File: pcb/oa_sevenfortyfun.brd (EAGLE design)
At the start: 88.9 x 63.4 mm, 45 parts, among them J1 1X01, J2 1X01, J3 1X01, J4 1X01, J5 1X01, J6 1X01, J7 1X01, J8 1X01, Q1 2N3904, Q10 2N3904, Q11 2N3904, Q12 2N3904, Q13 2N3904, Q14 2N3904, Q15 2N3906, Q16 2N3904, Q17 2N3906, Q18 2N3906, Q19 2N3906, Q2 2N3904, Q20 2N3906, Q3 2N3906, Q4 2N3906, Q5 2N3904, Q6 2N3904, Q7 2N3904, Q8 2N3904, Q9 2N3904

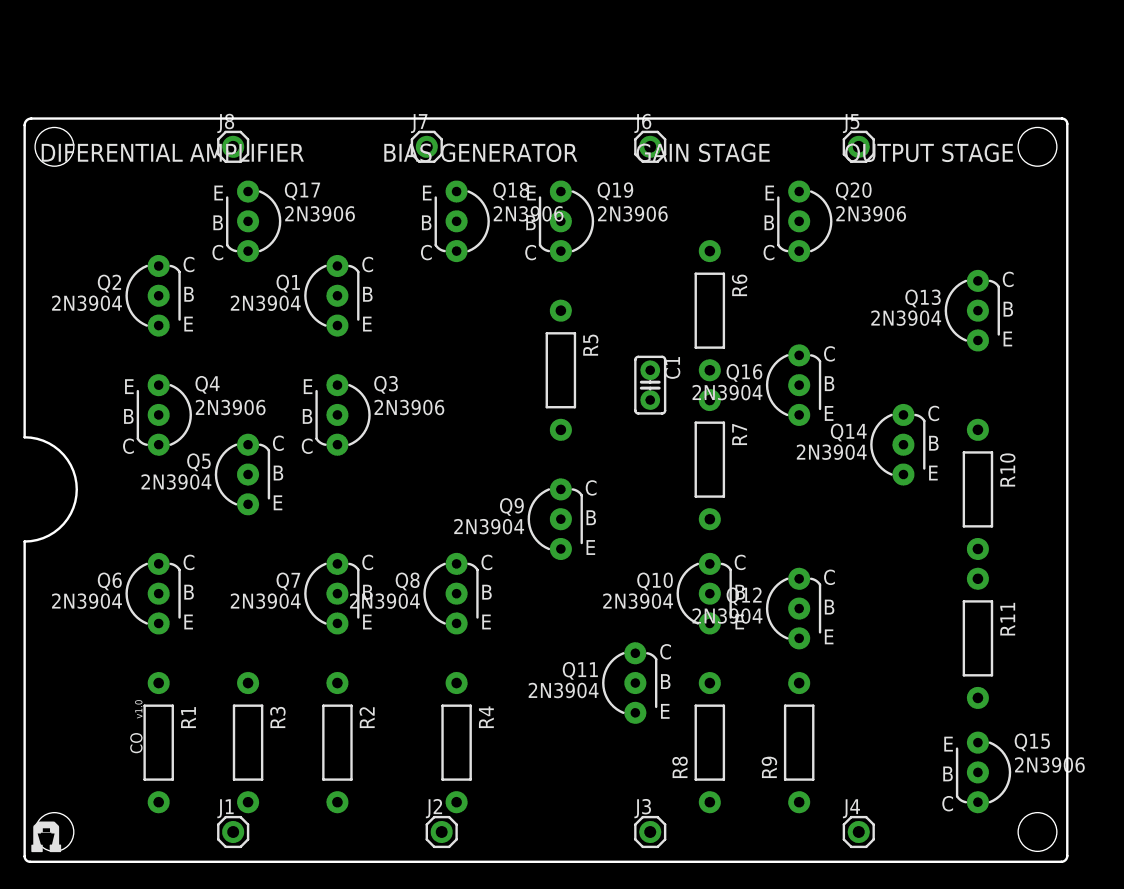
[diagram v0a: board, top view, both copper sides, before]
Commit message: Working on silkscreen
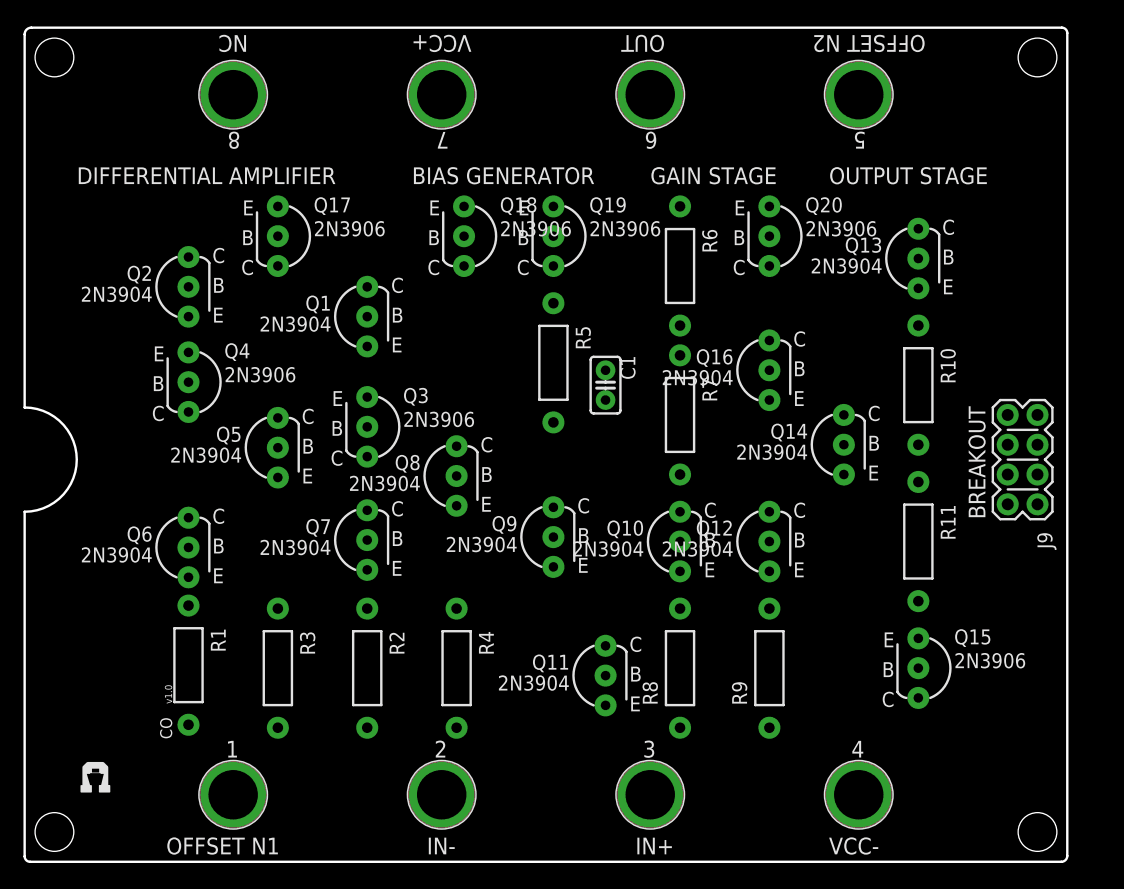
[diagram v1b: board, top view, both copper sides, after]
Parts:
- added J9: 2X04, Ai_Connectors:2X04
- J1, J2, J3, J4, J5, J6, J7, J8: value 1X01 -> 1X01-TERM; device Ai_Connectors:1X01 -> Ai_Connectors:1X01-TERM
- moved Q15 10.2 mm to (76.2, 16.5)
- moved R10 10.2 mm to (76.2, 40.6)
- moved Q8 10.0 mm to (36.8, 32.9)
- moved R11 9.69 mm to (76.2, 27.3)
- moved STANDOFF3 7.62 mm to (2.54, 68.6)
- moved STANDOFF4 7.62 mm to (86.4, 68.6)
- moved R1 7.08 mm to (14.0, 16.8)
- moved R9 6.84 mm to (63.5, 16.5)
- moved R2 6.84 mm to (29.2, 16.5)
- moved R3 6.84 mm to (21.6, 16.5)
- moved R8 6.84 mm to (55.9, 16.5)
- moved Q13 6.75 mm to (76.2, 51.4)
- moved U$3 6.59 mm to (4.70, 5.84)
- moved R4 6.35 mm to (36.8, 16.5)
- moved Q12 6.25 mm to (63.5, 27.3)
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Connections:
- net IN+: now also J9.5
- net IN-: now also J9.3
- net NC: now also J9.2
- net OFFSET_N1: now also J9.1
- net OFFSET_N2: now also J9.8
- net OUT: now also J9.6
- net VCC+: now also J9.4
- net VCC-: now also J9.7
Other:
- board size 88.9 x 63.4 mm -> 88.9 x 71.1 mm
- board text added: "1"
- board text added: "2"
- board text added: "3"
- board text added: "4"
- board text added: "5"
- board text added: "6"
- board text added: "7"
- board text added: "8"
- board text added: "BREAKOUT"
- board text added: "DIFFERENTIAL AMPLIFIER"
- board text added: "IN+"
- board text added: "IN-"
- board text added: "NC"
- board text added: "OFFSET N1"
- board text added: "OFFSET N2"
- board text added: "OUT"
- board text added: "VCC+"
- board text added: "VCC-"
- board text removed: "DIFERENTIAL AMPLIFIER"

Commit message: Working on silkscreen
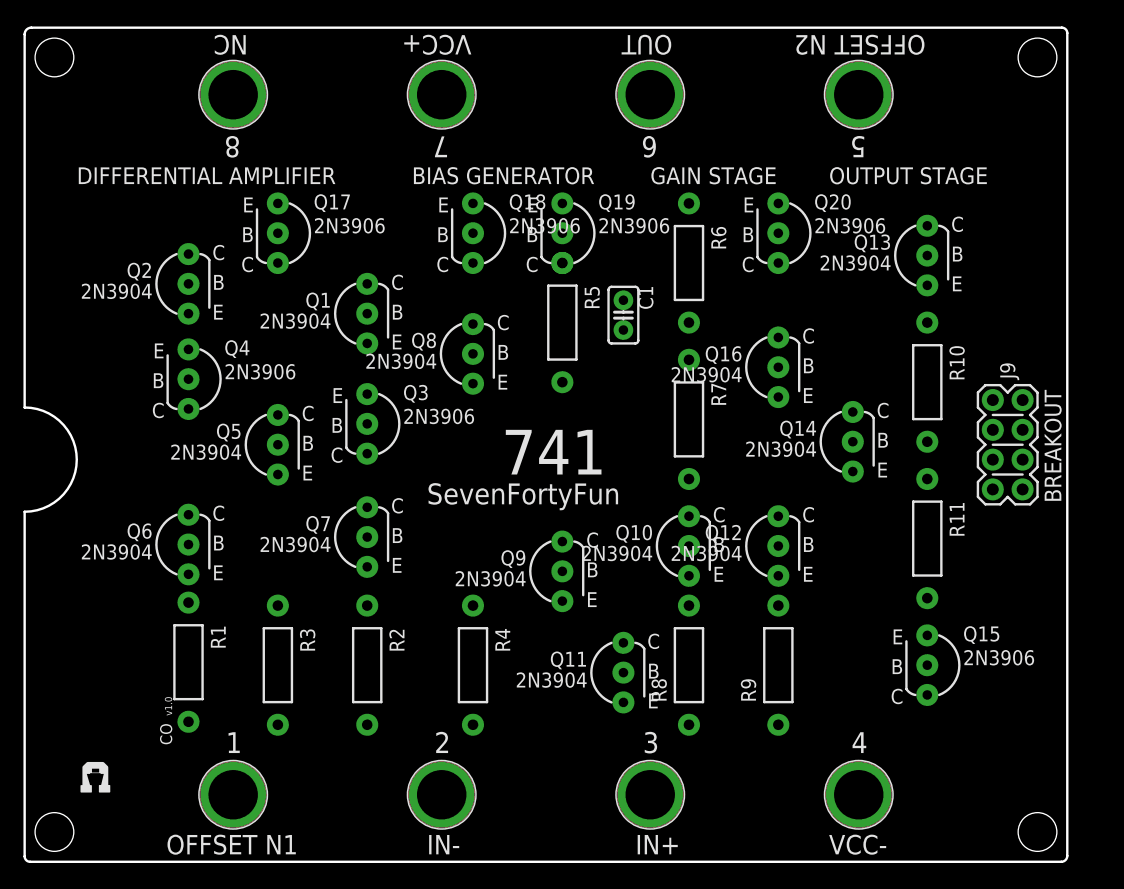
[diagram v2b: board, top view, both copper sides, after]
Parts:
- moved Q8 10.5 mm to (38.2, 43.3)
- moved C1 6.16 mm to (51.1, 46.6)
- moved R5 3.51 mm to (45.8, 46.0)
- moved Q9 3.02 mm to (45.8, 24.8)
- moved J9 1.80 mm to (83.8, 35.6)
- moved Q11 1.55 mm to (51.1, 16.1)
- moved R4 1.42 mm to (38.2, 16.8)
- moved Q10 0.85 mm to (56.6, 26.9)
- moved Q12 0.85 mm to (64.3, 26.9)
- moved R7 0.85 mm to (56.6, 37.7)
- moved Q16 0.80 mm to (64.3, 42.2)
- moved R6 0.80 mm to (56.6, 51.1)
- moved R11 0.80 mm to (77.0, 27.6)
- moved Q13 0.80 mm to (77.0, 51.7)
- moved Q14 0.80 mm to (70.6, 35.8)
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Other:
- board text added: "741"
- board text added: "SevenFortyFun"
